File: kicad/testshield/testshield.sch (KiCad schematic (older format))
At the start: 6 parts, among them J1 ISP header, J2 Raspiheader, SW1 SW_Push, U1 ATMEGA328P-PU

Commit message: update
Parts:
- R1: footprint Resistors_THT:R_Axial_DIN0207_L6.3mm_D2.5mm_P10.16mm_Horizontal -> Resistors_SMD:R_2010
- U1: footprint ATMEGA328P-PU:DIP794W46P254L2967H457Q28B -> ATMEGA328P-AU:QFP80P900X900X120-32N
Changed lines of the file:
@@
 F 0 "U1" H 3200 4600 50  0000 L BNN
 F 1 "ATMEGA328P-PU" H 4350 1950 50  0000 L BNN
-F 2 "ATMEGA328P-PU:DIP794W46P254L2967H457Q28B" H 3950 3350 50  0001 C CIN
+F 2 "ATMEGA328P-AU:QFP80P900X900X120-32N" H 3950 3350 50  0001 C CIN
 F 3 "" H 3950 3350 50  0001 C CNN
 	1    3950 3350
@@
 F 0 "R1" V 6130 3250 50  0000 C CNN
 F 1 "10k" V 6050 3250 50  0000 C CNN
-F 2 "Resistors_THT:R_Axial_DIN0207_L6.3mm_D2.5mm_P10.16mm_Horizontal" V 5980 3250 50  0001 C CNN
+F 2 "Resistors_SMD:R_2010" V 5980 3250 50  0001 C CNN
 F 3 "" H 6050 3250 50  0001 C CNN
 	1    6050 3250

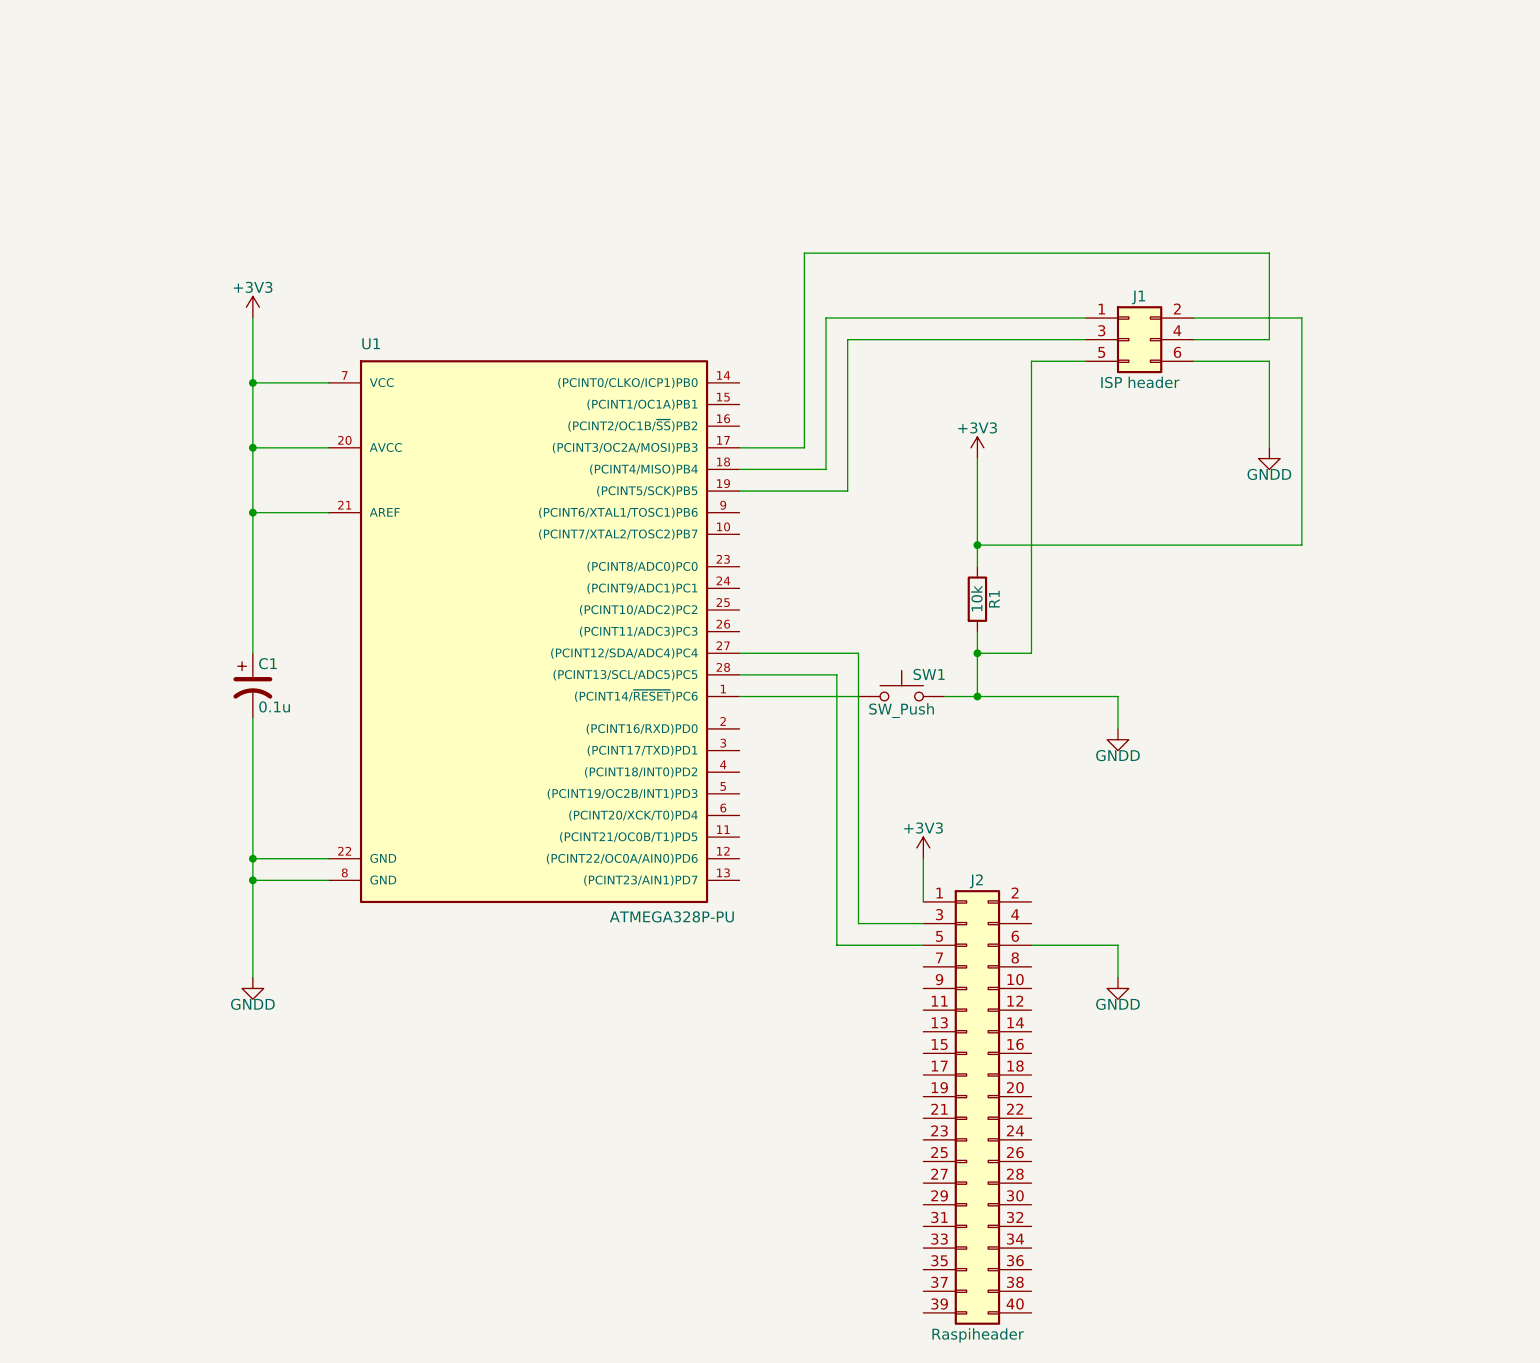
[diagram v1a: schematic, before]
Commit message: Add files via upload
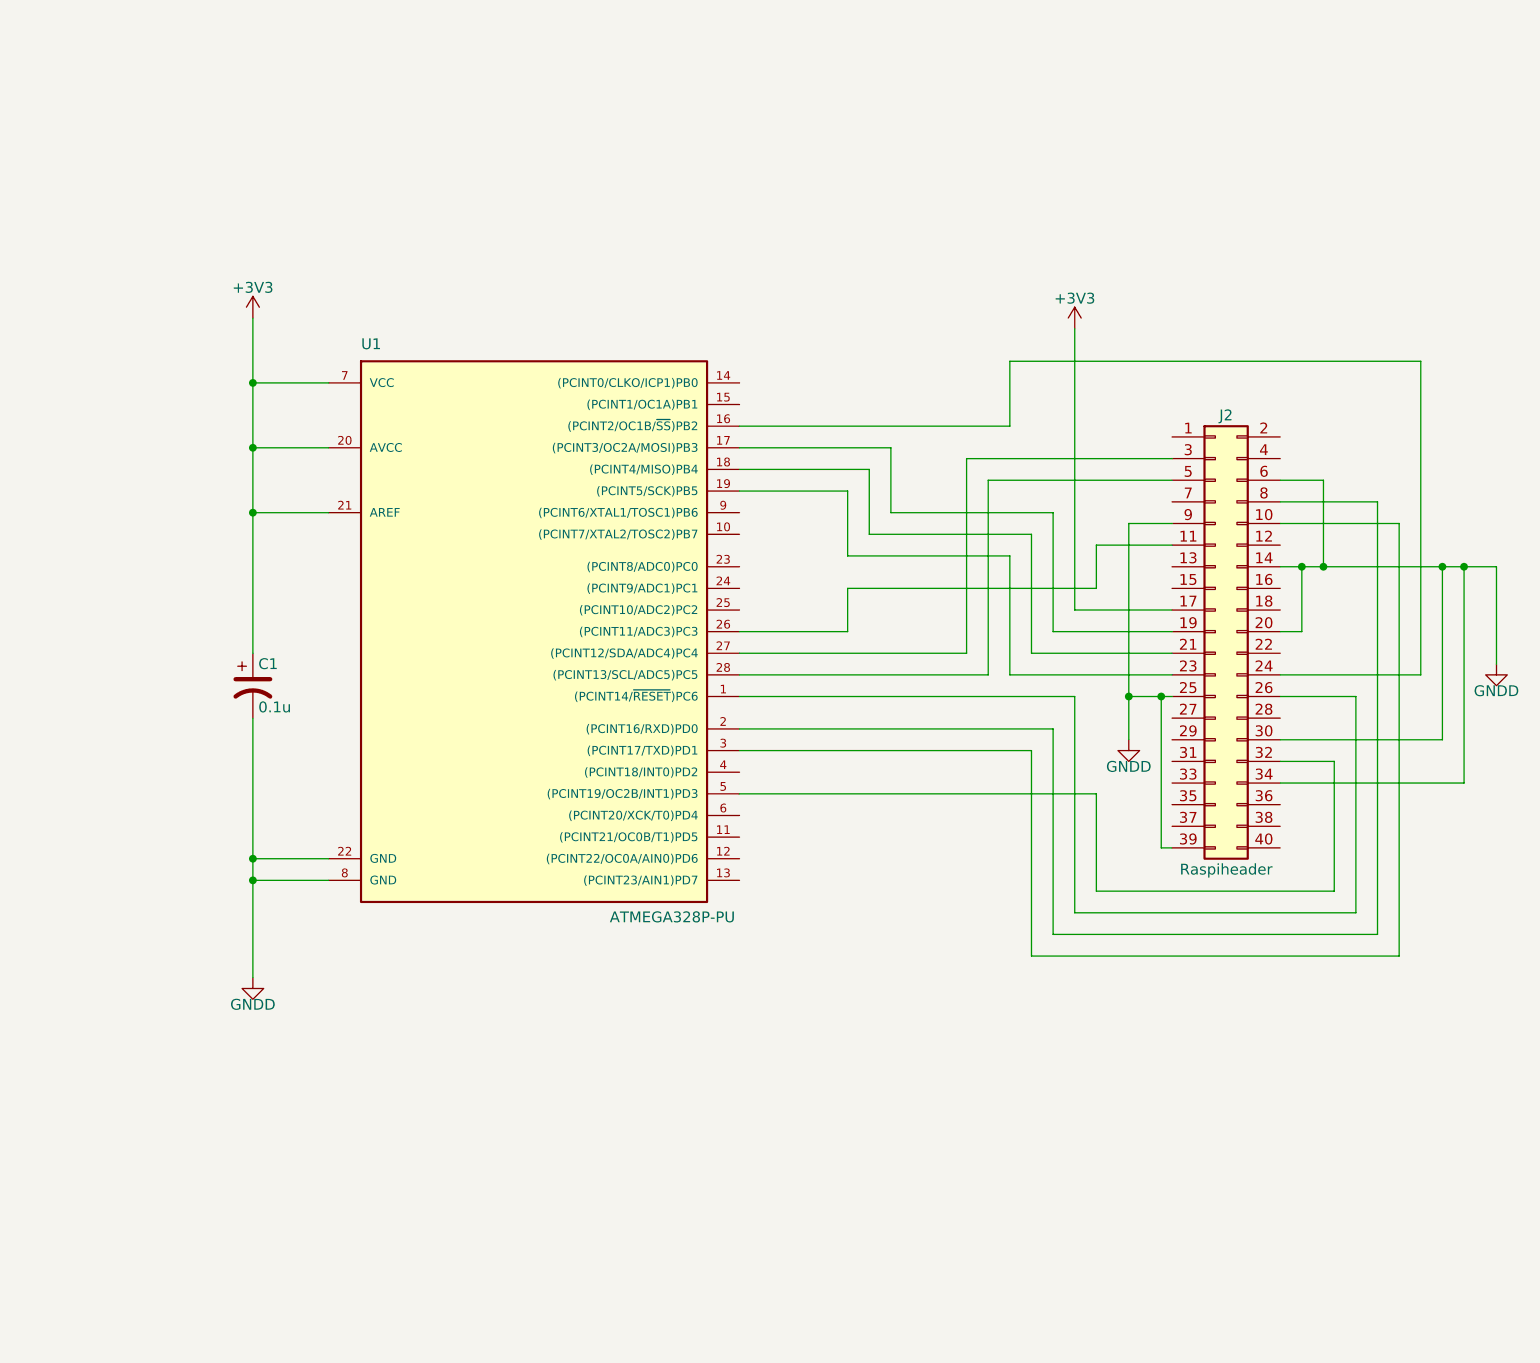
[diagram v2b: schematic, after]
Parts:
- removed J1: ISP header, Pin_Headers:Pin_Header_Straight_2x03_Pitch2.54mm, symbol Conn_02x03_Odd_Even
- removed R1: 10k, Resistors_SMD:R_2010, symbol R
- removed SW1: SW_Push, Buttons_Switches_SMD:SW_SPST_B3S-1000, symbol SW_Push
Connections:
- net +3V3: now also J2.17 (Pin_17); no longer J2.1 (Pin_1)
- net GNDD: now also J2.14 (Pin_14), J2.20 (Pin_20), J2.25 (Pin_25), J2.30 (Pin_30), J2.34 (Pin_34), J2.39 (Pin_39), J2.9 (Pin_9)
- net at U1.1 ((PCINT14/~RESET~)PC6): now also J2.26 (Pin_26)
- net at U1.16 ((PCINT2/OC1B/~SS~)PB2): now also J2.24 (Pin_24)
- net at U1.17 ((PCINT3/OC2A/MOSI)PB3): now also J2.19 (Pin_19)
- net at U1.18 ((PCINT4/MISO)PB4): now also J2.21 (Pin_21)
- net at U1.19 ((PCINT5/SCK)PB5): now also J2.23 (Pin_23)
- net at U1.2 ((PCINT16/RXD)PD0): now also J2.8 (Pin_8)
- net at U1.26 ((PCINT11/ADC3)PC3): now also J2.11 (Pin_11)
- net at U1.3 ((PCINT17/TXD)PD1): now also J2.10 (Pin_10)
- net at U1.5 ((PCINT19/OC2B/INT1)PD3): now also J2.32 (Pin_32)
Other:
- moved on the sheet: J2

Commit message: Add files via upload
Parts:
- added D1: LED1, LEDs:LED_0603, symbol LED
- added D2: LED2, LEDs:LED_0603, symbol LED
- added J1: ISP/PDI, Pin_Headers:Pin_Header_Straight_2x03_Pitch2.54mm, symbol Conn_02x03_Odd_Even
- added R1: 1k, Resistors_SMD:R_0603, symbol R
- added R2, R3: 330, Resistors_SMD:R_0603, symbol R
- added R4: 10k, Resistors_SMD:R_0603, symbol R
- added SW1: Reset, Buttons_Switches_SMD:SW_SPST_B3U-1000P, symbol SW_Push
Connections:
- wire segments 75 -> 99
